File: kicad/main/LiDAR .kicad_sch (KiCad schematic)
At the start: 5 parts, among them Q20 AO3400

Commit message: Fix edge cut; no-CM STEP
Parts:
- R47: footprint Resistor_SMD:R_0603_1608Metric_Pad0.98x0.95mm_HandSolder -> Resistor_SMD:R_0603_1608Metric
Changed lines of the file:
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@@
 		)
 		(instances
-			(project "oomwoo-kicad"
+			(project "Main"
 				(path "/dbcfb655-8d45-4808-9a74-2a0eb03372e8/994d55da-8e8c-4fe8-9877-f2e4533982e7"
 					(reference "Q20")
@@
 		)
 		(instances
-			(project "oomwoo-kicad"
+			(project "Main"
 				(path "/dbcfb655-8d45-4808-9a74-2a0eb03372e8/994d55da-8e8c-4fe8-9877-f2e4533982e7"
 					(reference "#PWR0600")
@@
 		)
 		(instances
-			(project "oomwoo-kicad"
+			(project "Main"
 				(path "/dbcfb655-8d45-4808-9a74-2a0eb03372e8/994d55da-8e8c-4fe8-9877-f2e4533982e7"
 					(reference "#PWR0603")
@@
 		)
 		(instances
-			(project "oomwoo-kicad"
+			(project "Main"
 				(path "/dbcfb655-8d45-4808-9a74-2a0eb03372e8/994d55da-8e8c-4fe8-9877-f2e4533982e7"
 					(reference "#PWR0605")
@@
 		)
 		(instances
-			(project "oomwoo-kicad"
+			(project "Main"
 				(path "/dbcfb655-8d45-4808-9a74-2a0eb03372e8/994d55da-8e8c-4fe8-9877-f2e4533982e7"
 					(reference "R116")
@@
 		)
 		(instances
-			(project "oomwoo-kicad"
+			(project "Main"
 				(path "/dbcfb655-8d45-4808-9a74-2a0eb03372e8/994d55da-8e8c-4fe8-9877-f2e4533982e7"
 					(reference "LIDAR1")
@@
 		)
 		(instances
-			(project "oomwoo-kicad"
+			(project "Main"
 				(path "/dbcfb655-8d45-4808-9a74-2a0eb03372e8/994d55da-8e8c-4fe8-9877-f2e4533982e7"
 					(reference "#PWR070")
@@
 			)
 		)
-		(property "Footprint" "Resistor_SMD:R_0603_1608Metric_Pad0.98x0.95mm_HandSolder"
+		(property "Footprint" "Resistor_SMD:R_0603_1608Metric"
 			(at 266.319 160.909 90)
 			(hide yes)
@@
 		)
 		(instances
-			(project "oomwoo-kicad"
+			(project "Main"
 				(path "/dbcfb655-8d45-4808-9a74-2a0eb03372e8/994d55da-8e8c-4fe8-9877-f2e4533982e7"
 					(reference "R47")
@@
 		)
 		(instances
-			(project "oomwoo-kicad"
+			(project "Main"
 				(path "/dbcfb655-8d45-4808-9a74-2a0eb03372e8/994d55da-8e8c-4fe8-9877-f2e4533982e7"
 					(reference "#PWR071")
@@
 		)
 		(instances
-			(project "oomwoo-kicad"
+			(project "Main"
 				(path "/dbcfb655-8d45-4808-9a74-2a0eb03372e8/994d55da-8e8c-4fe8-9877-f2e4533982e7"
 					(reference "D10")

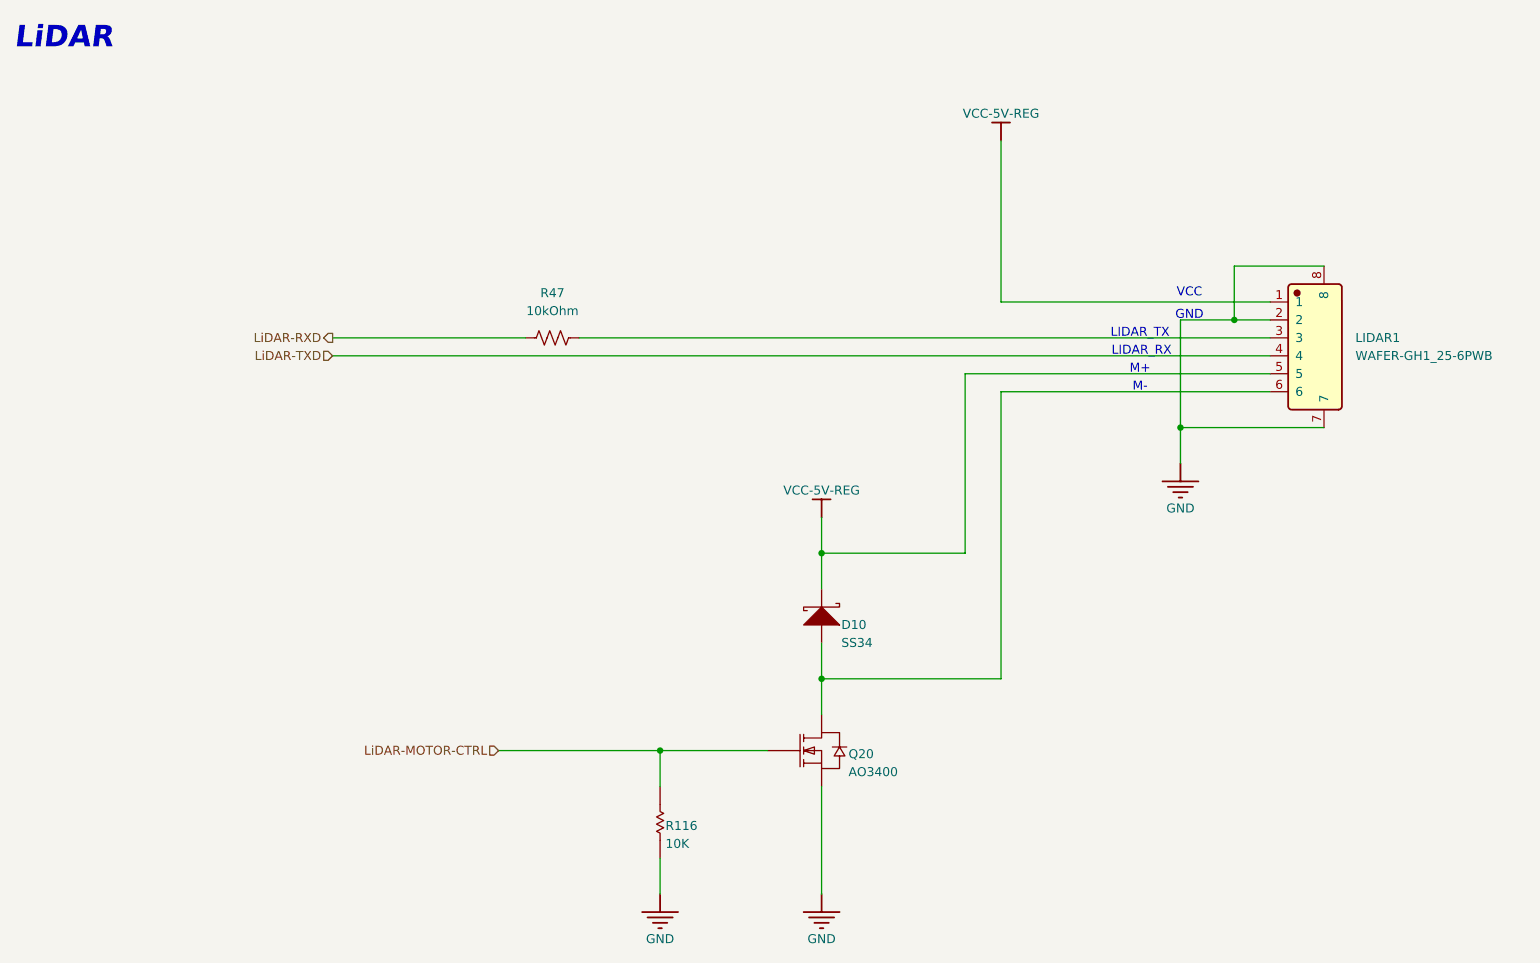
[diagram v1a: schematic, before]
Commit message: Schematic fixes, 1st round of review
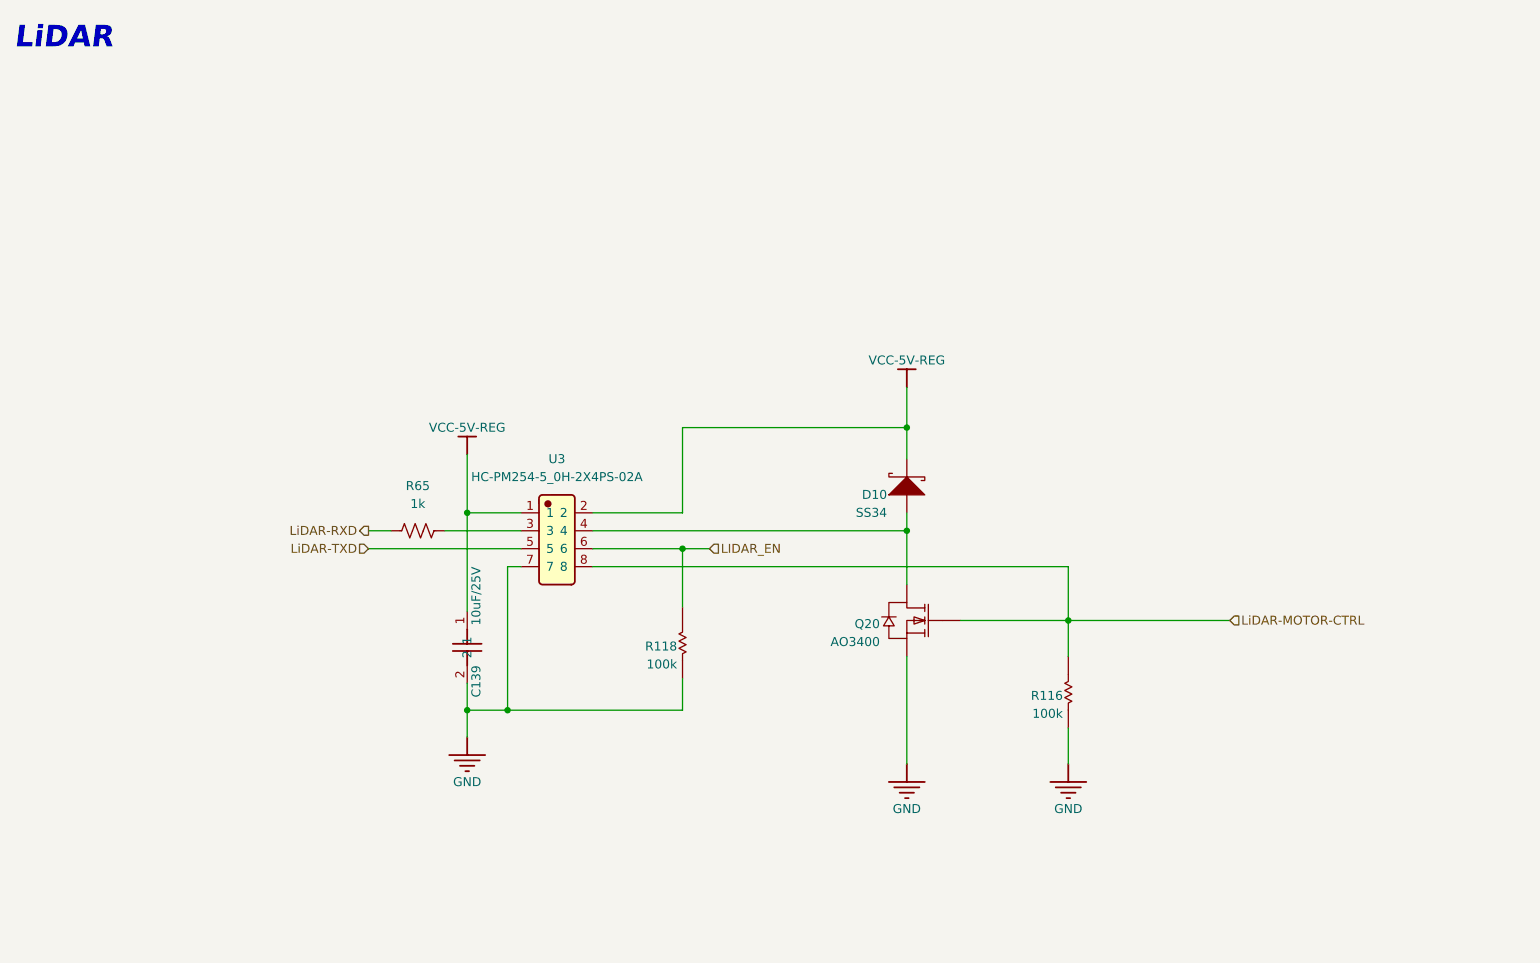
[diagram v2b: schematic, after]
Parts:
- removed LIDAR1: WAFER-GH1_25-6PWB, JLCImport:WAFER-GH1_25-6PWB, symbol JLCImport:WAFER-GH1_25-6PWB
- removed R47: 10kOhm, Resistor_SMD:R_0603_1608Metric, symbol Device:R_US
- added C139: 10uF/25V, Capacitor_SMD:C_0603_1608Metric, symbol JLCImport:CL21A106KBYQNNE
- added R118: 100k, Resistor_SMD:R_0603_1608Metric, symbol DesignLibrary:LiDAR_1_Resistor-1_DesignLibrary.SchLib
- added R65: 1k, Resistor_SMD:R_0603_1608Metric, symbol Device:R_US
- added U3: HC-PM254-5_0H-2X4PS-02A, JLCImport:HC-PM254-5_0H-2X4PS-02A, symbol JLCImport:HC-PM254-5_0H-2X4PS-02A
- D10: footprint oomwoo_altium:SMA -> Diode_SMD:D_SMA; LCSC (none) -> C22448055; MANUFACTURER * -> (none); Manufacturer (none) -> *
- Q20: LCSC (none) -> C20628874; MANUFACTURER * -> (none); Manufacturer (none) -> *
- R116: value 10K -> 100k; MANUFACTURER * -> (none); Manufacturer (none) -> *
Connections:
- net GND: now also C139.2, R118.1, U3.7
- net LiDAR-MOTOR-CTRL: now also U3.8
- net LiDAR-RXD: now also R65.1
- net LiDAR-TXD: now also U3.5
- net VCC-5V-REG: now also C139.1, U3.1, U3.2
- net at D10.1 (A), Q20.3 (D): now also U3.4
- new net: R65.2, U3.3
- new net LIDAR_EN: R118.2, U3.6
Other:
- note removed: "GND"
- note removed: "LIDAR_RX"
- note removed: "LIDAR_TX"
- note removed: "M+"
- note removed: "M-"
- note removed: "VCC"
- moved on the sheet: D10, Q20, R116
